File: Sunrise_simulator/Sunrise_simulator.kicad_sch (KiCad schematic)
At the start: 21 parts, among them J1 Jack-DC, J2 SD_Card_Device, Q1 BS170, SW1 Switch ON-OFF, SW2 BUTTON_PLUS, SW3 BUTTON_MINUS, SW4 BUTTON_VALIDATE, SW5 BUTTON_PARAMETER, U1 MP1584EN, U2 MAX98357A, U3 E-ink display, U4 DS3231MZ

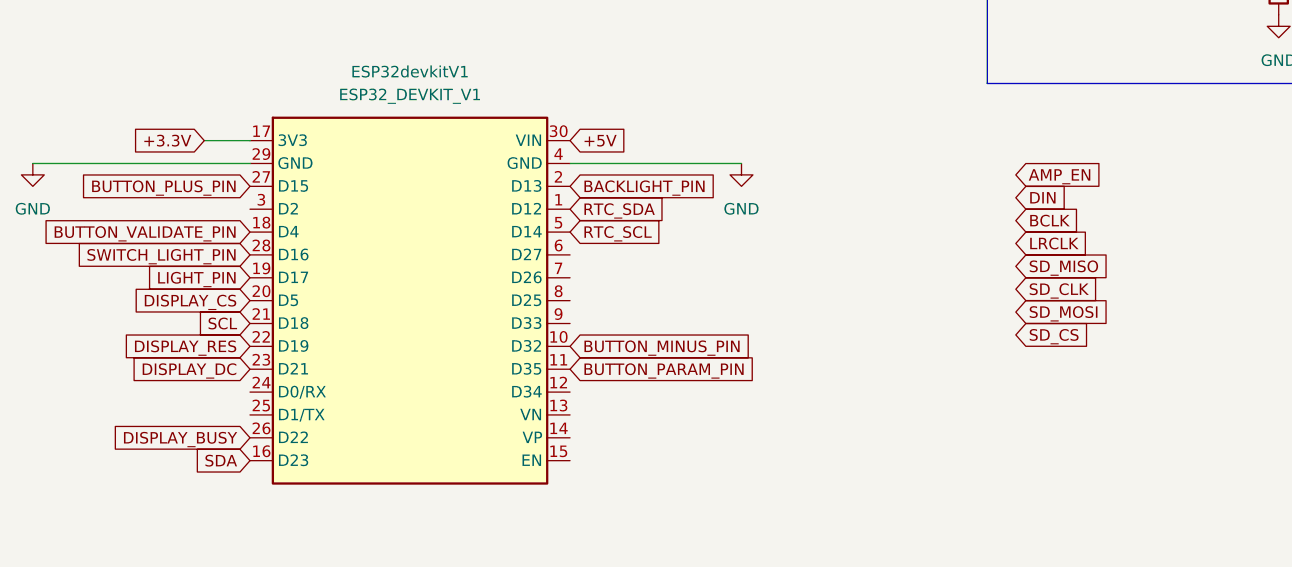
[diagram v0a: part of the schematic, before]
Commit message: update kicad schematic
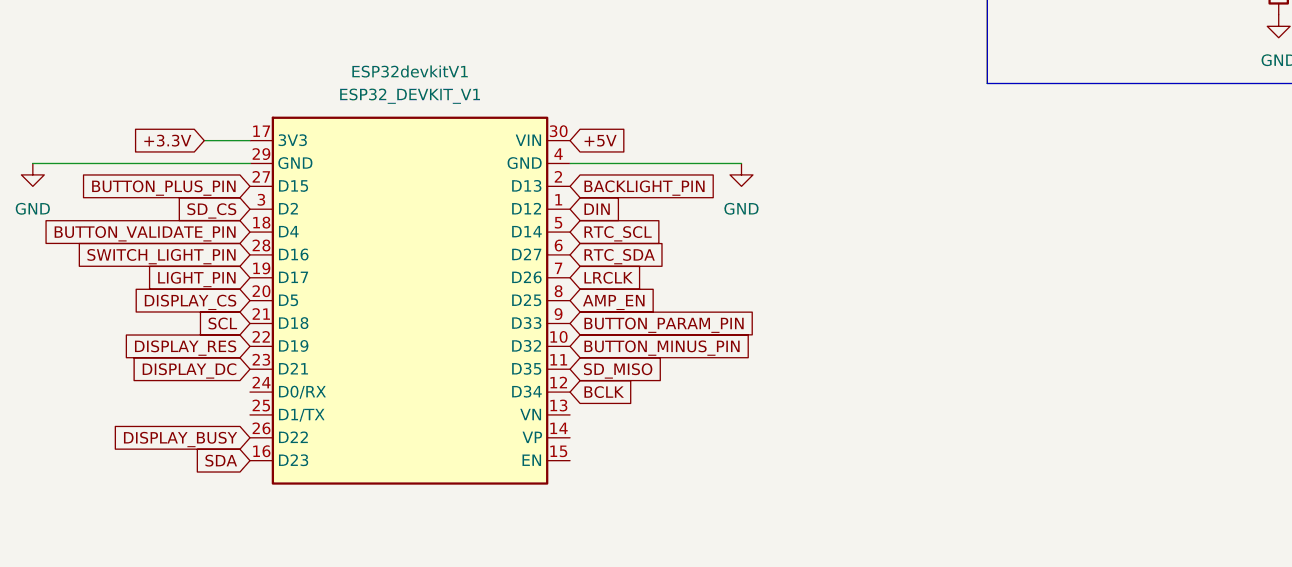
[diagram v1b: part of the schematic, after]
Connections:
- net AMP_EN: now also ESP32devkitV1.8 (D25)
- net BCLK: now also ESP32devkitV1.12 (D34)
- net BUTTON_PARAM_PIN: now also ESP32devkitV1.9 (D33); no longer ESP32devkitV1.11 (D35)
- net DIN: now also ESP32devkitV1.1 (D12)
- net LRCLK: now also ESP32devkitV1.7 (D26)
- net RTC_SDA: now also ESP32devkitV1.6 (D27); no longer ESP32devkitV1.1 (D12)
- net SD_CS: now also ESP32devkitV1.3 (D2)
- net SD_MISO: now also ESP32devkitV1.11 (D35)
